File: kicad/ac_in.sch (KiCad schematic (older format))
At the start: 32 parts, among them J701 tblock, U702 R-783.3-1.0, U704 R-78E5.0-1.0, U705 AP2114H-1.2TRG1, U706 AP2114H-1.2TRG1

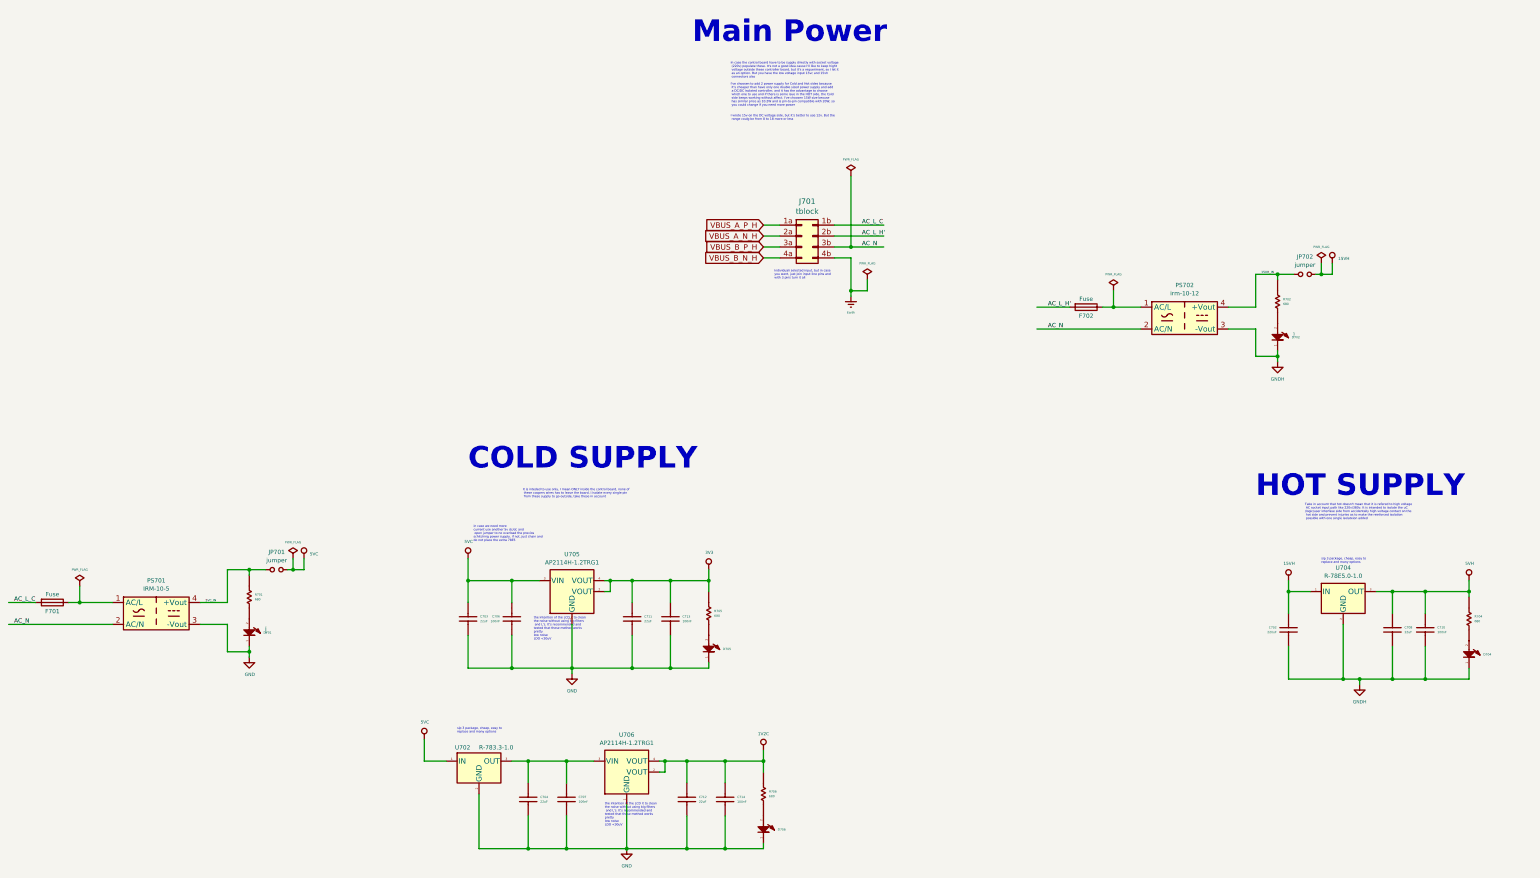
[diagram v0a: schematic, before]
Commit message: beginine routing... far far away
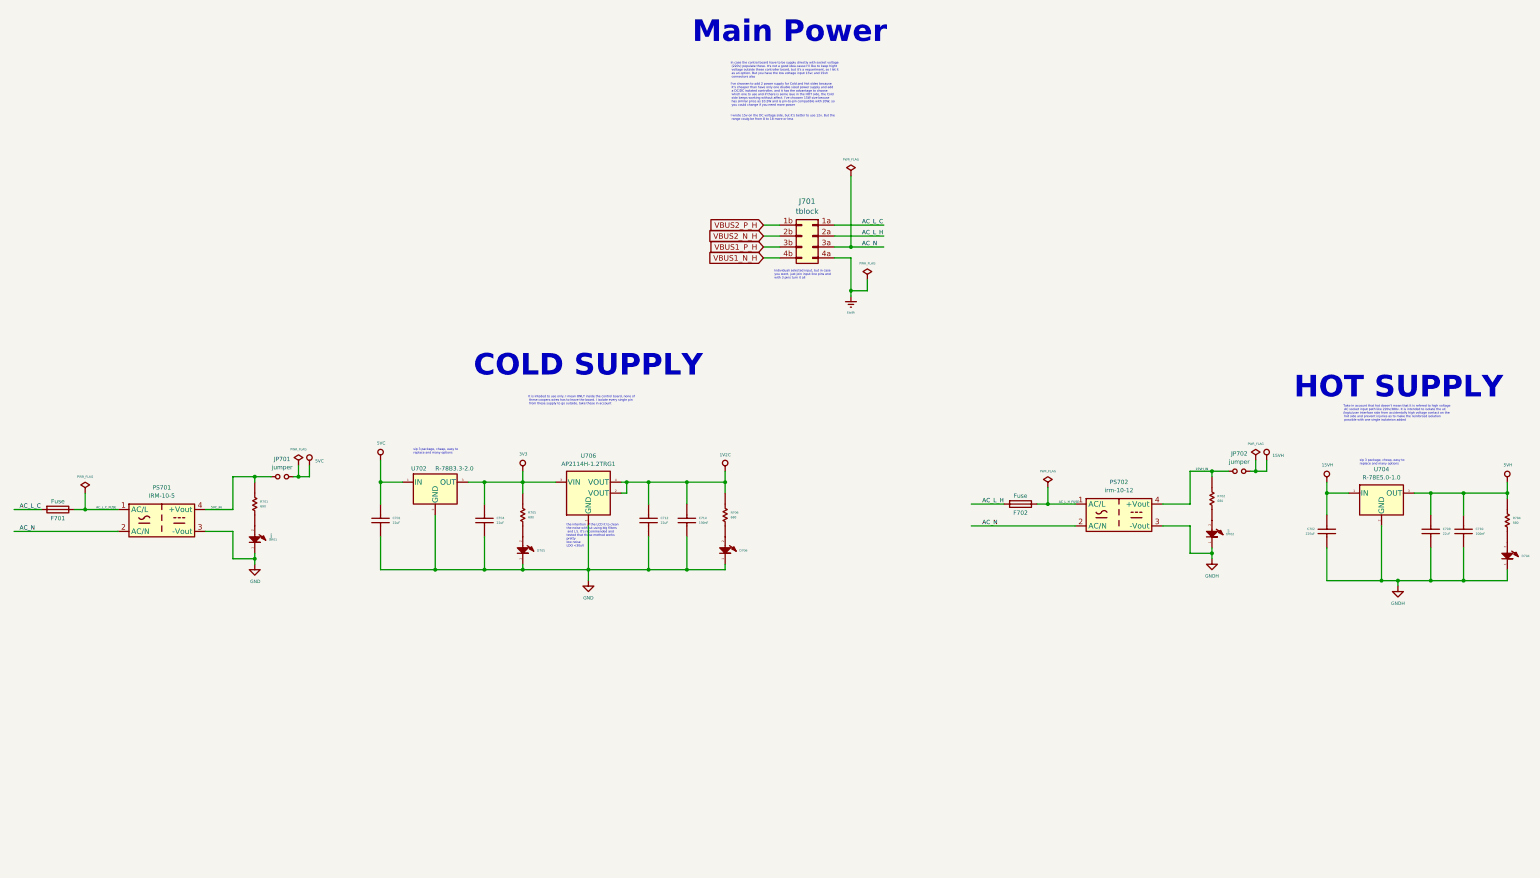
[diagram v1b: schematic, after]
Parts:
- removed C703, C711: 22uF, servo:C_0603_1608Metric, symbol servo:Capacitor
- removed C706, C707, C713: 100nF, servo:C_0603_1608Metric, symbol servo:Capacitor
- removed U705: AP2114H-1.2TRG1, Package_TO_SOT_SMD:SOT-223, symbol servo:AP2114
- added C701: 22uF, servo:C_0603_1608Metric, symbol servo:Capacitor
- U702: value R-783.3-1.0 -> R-78B3.3-2.0
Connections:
- net labels added: AC_L_C_FUSE, AC_L_H, AC_L_H_FUSE, VBUS1_N_H, VBUS1_P_H, VBUS2_N_H, VBUS2_P_H
- net labels removed: AC_L_H', VBUS_A_N_H, VBUS_A_P_H, VBUS_B_N_H, VBUS_B_P_H
- wire segments 130 -> 108
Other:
- note removed: "in case we need more \ncurrent use another 5v dc/dc and\n open jumper to no overload the previos \nschitching power supply. if not, just chain and \ndo not place the extra 78E5"
- moved on the sheet: C702, C704, C708, C710, C712, C714, D701, D702, D704, D705, D706, F701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

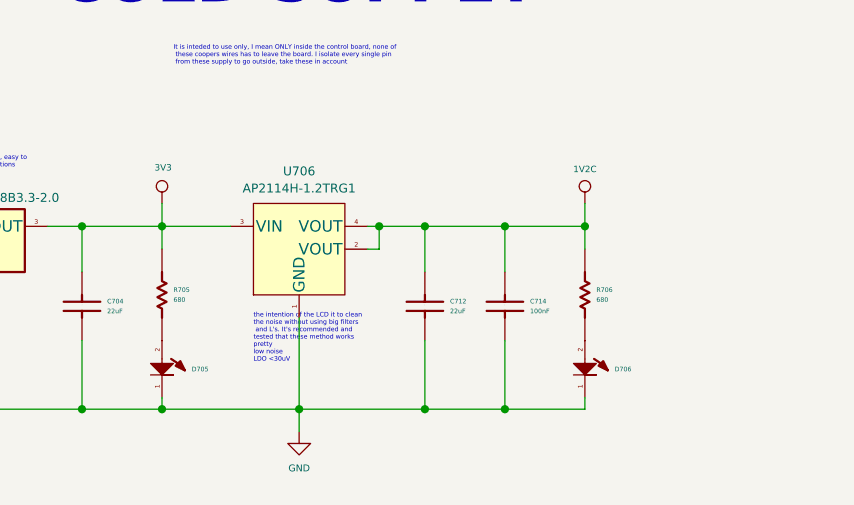
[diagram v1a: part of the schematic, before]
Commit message: touting....
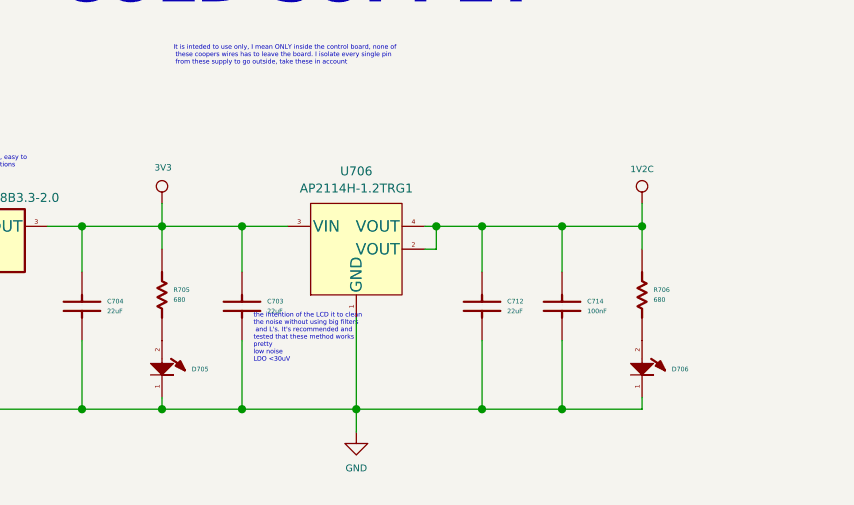
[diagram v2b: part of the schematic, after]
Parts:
- added C703: 22uF, servo:C_0603_1608Metric, symbol servo:Capacitor
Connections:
- wire segments 108 -> 112
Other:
- moved on the sheet: C712, C714, D706, R706, U706
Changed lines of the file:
@@
 L servo:1V2C #PWR0719
 U 1 1 5DDC3F59
-P 7850 5550
-F 0 "#PWR0719" H 7850 5350 20  0001 C CNN
-F 1 "1V2C" H 7850 5700 28  0000 C CNN
-F 2 "" H 7850 5550 50  0001 C CNN
-F 3 "" H 7850 5550 50  0001 C CNN
-	1    7850 5550
+P 8100 5550
+F 0 "#PWR0719" H 8100 5350 20  0001 C CNN
+F 1 "1V2C" H 8100 5700 28  0000 C CNN
+F 2 "" H 8100 5550 50  0001 C CNN
+F 3 "" H 8100 5550 50  0001 C CNN
+	1    8100 5550
 	1    0    0    -1
 $EndComp
@@
 	5200 5950 5200 6450
 Wire Wire Line
-	7850 5650 7850 5550
-Wire Wire Line
-	7850 5650 7850 5750
-Connection ~ 7850 5650
+	8100 5650 8100 5550
+Wire Wire Line
+	8100 5650 8100 5750
+Connection ~ 8100 5650
 $Comp
 L servo:Resistor R?
 U 1 1 5E18DDBA
-P 7850 5950
+P 8100 5950
 AR Path="/5EAA846A/5E18DDBA" Ref="R?"  Part="1"
 AR Path="/5DD76B18/5E18DDBA" Ref="R706"  Part="1"
-F 0 "R706" V 7828 6000 20  0000 L CNN
-F 1 "680" V 7871 6000 20  0000 L CNN
-F 2 "Resistor_SMD:R_0603_1608Metric" H 7350 5850 60  0001 C CNN
-F 3 "" H 7450 5950 60  0001 C CNN
-F 4 "680" V -4550 6350 60  0001 C CNN "ValueDisplayed"
-	1    7850 5950
+F 0 "R706" V 8078 6000 20  0000 L CNN
+F 1 "680" V 8121 6000 20  0000 L CNN
+F 2 "Resistor_SMD:R_0603_1608Metric" H 7600 5850 60  0001 C CNN
+F 3 "" H 7700 5950 60  0001 C CNN
+F 4 "680" V -4300 6350 60  0001 C CNN "ValueDisplayed"
+	1    8100 5950
 	0    1    1    0
 $EndComp
@@
 L servo:LED_A2_K1 D?
 U 1 1 5E18DDBB
-P 7850 6250
+P 8100 6250
 AR Path="/5EAA846A/5E18DDBB" Ref="D?"  Part="1"
 AR Path="/5DD76B18/5E18DDBB" Ref="D706"  Part="1"
-F 0 "D706" V 7875 6380 20  0000 L CNN
-F 1 "blue" H 7850 6400 16  0001 C CNN
-F 2 "servo:LED_0603_1608Metric" H 7650 6050 60  0001 C CNN
-F 3 "" H 7650 6050 60  0000 C CNN
-F 4 "red" V -4550 6150 60  0001 C CNN "VALUE"
-	1    7850 6250
-	0    1    1    0
-$EndComp
-Wire Wire Line
-	7850 6400 7850 6450
+F 0 "D706" V 8125 6380 20  0000 L CNN
+F 1 "blue" H 8100 6400 16  0001 C CNN
+F 2 "servo:LED_0603_1608Metric" H 7900 6050 60  0001 C CNN
+F 3 "" H 7900 6050 60  0000 C CNN
+F 4 "red" V -4300 6150 60  0001 C CNN "VALUE"
+	1    8100 6250
+	0    1    1    0
+$EndComp
+Wire Wire Line
+	8100 6400 8100 6450
 $Comp
 L servo:GND #PWR?
 U 1 1 5E286204
-P 6600 6550
+P 6850 6550
 AR Path="/5DCD812E/5E286204" Ref="#PWR?"  Part="1"
 AR Path="/5EAA846A/5E286204" Ref="#PWR?"  Part="1"
 AR Path="/5DD76B18/5E286204" Ref="#PWR0715"  Part="1"
-F 0 "#PWR0715" H 6605 6401 20  0001 C CNN
-F 1 "GND" H 6600 6392 30  0000 C CNN
-F 2 "" H 6600 6550 70  0000 C CNN
-F 3 "" H 6600 6550 70  0000 C CNN
-	1    6600 6550
+F 0 "#PWR0715" H 6855 6401 20  0001 C CNN
+F 1 "GND" H 6850 6392 30  0000 C CNN
+F 2 "" H 6850 6550 70  0000 C CNN
+F 3 "" H 6850 6550 70  0000 C CNN
+	1    6850 6550
 	1    0    0    -1
 $EndComp
@@
 L servo:Capacitor C?
 U 1 1 5E28620B
-P 7150 5950
+P 7400 5950
 AR Path="/5EAA846A/5E28620B" Ref="C?"  Part="1"
 AR Path="/5DD76B18/5E28620B" Ref="C712"  Part="1"
-F 0 "C712" V 7178 6060 20  0000 L CNN
-F 1 "22uF" V 7221 6060 20  0000 L CNN
-F 2 "servo:C_0603_1608Metric" H 7150 5850 60  0001 C CNN
-F 3 "" H 7150 5950 60  0000 C CNN
-F 4 "22uF" V -5850 6350 60  0001 C CNN "ValueDisplayed"
-	1    7150 5950
+F 0 "C712" V 7428 6060 20  0000 L CNN
+F 1 "22uF" V 7471 6060 20  0000 L CNN
+F 2 "servo:C_0603_1608Metric" H 7400 5850 60  0001 C CNN
+F 3 "" H 7400 5950 60  0000 C CNN
+F 4 "22uF" V -5600 6350 60  0001 C CNN "ValueDisplayed"
+	1    7400 5950
 	0    1    1    0
 $EndComp
@@
 L servo:Capacitor C?
 U 1 1 5E286219
-P 7500 5950
+P 7750 5950
 AR Path="/5EAA846A/5E286219" Ref="C?"  Part="1"
 AR Path="/5DD76B18/5E286219" Ref="C714"  Part="1"
-F 0 "C714" V 7528 6060 20  0000 L CNN
-F 1 "100nF" V 7571 6060 20  0000 L CNN
-F 2 "servo:C_0603_1608Metric" H 7500 5850 60  0001 C CNN
-F 3 "" H 7500 5950 60  0000 C CNN
-F 4 "22uF" V -5500 6350 60  0001 C CNN "ValueDisplayed"
-	1    7500 5950
+F 0 "C714" V 7778 6060 20  0000 L CNN
+F 1 "100nF" V 7821 6060 20  0000 L CNN
+F 2 "servo:C_0603_1608Metric" H 7750 5850 60  0001 C CNN
+F 3 "" H 7750 5950 60  0000 C CNN
+F 4 "22uF" V -5250 6350 60  0001 C CNN "ValueDisplayed"
+	1    7750 5950
 	0    1    1    0
 $EndComp
@@
 HOT SUPPLY
 Wire Wire Line
-	6900 5650 6950 5650
-Wire Wire Line
-	6900 5750 6950 5750
-Wire Wire Line
-	6950 5750 6950 5650
-Connection ~ 6950 5650
-Wire Wire Line
-	6600 6050 6600 6450
-Connection ~ 6600 6450
+	7150 5650 7200 5650
+Wire Wire Line
+	7150 5750 7200 5750
+Wire Wire Line
+	7200 5750 7200 5650
+Connection ~ 7200 5650
+Wire Wire Line
+	6850 6050 6850 6450
+Connection ~ 6850 6450
 Connection ~ 15000 5750
 Wire Wire Line
@@
 	5500 5650 5650 5650
 Wire Wire Line
-	6950 5650 7150 5650
+	7200 5650 7400 5650
 Wire Wire Line
 	5650 5850 5650 5650
@@
 L servo:AP2114 U706
 U 1 1 5E28622B
-P 6600 5750
-F 0 "U706" H 6600 6091 39  0000 C CNN
-F 1 "AP2114H-1.2TRG1" H 6600 6016 39  0000 C CNN
-F 2 "Package_TO_SOT_SMD:SOT-223" H 6700 6375 50  0001 C CNN
-F 3 "../doc/datasheets/AP2114.pdf" H 6650 6150 50  0001 C CNN
-	1    6600 5750
-	1    0    0    -1
-$EndComp
-Wire Wire Line
-	7150 6150 7150 6450
-Wire Wire Line
-	6600 6450 7150 6450
-Connection ~ 7150 6450
-Wire Wire Line
-	7150 6450 7500 6450
-Wire Wire Line
-	7500 6150 7500 6450
-Connection ~ 7500 6450
-Wire Wire Line
-	7500 6450 7850 6450
-Wire Wire Line
-	7150 5850 7150 5650
-Connection ~ 7150 5650
-Wire Wire Line
-	7500 5850 7500 5650
-Wire Wire Line
-	7150 5650 7500 5650
-Connection ~ 7500 5650
-Wire Wire Line
-	7500 5650 7850 5650
+P 6850 5750
+F 0 "U706" H 6850 6091 39  0000 C CNN
+F 1 "AP2114H-1.2TRG1" H 6850 6016 39  0000 C CNN
+F 2 "Package_TO_SOT_SMD:SOT-223" H 6950 6375 50  0001 C CNN
+F 3 "../doc/datasheets/AP2114.pdf" H 6900 6150 50  0001 C CNN
+	1    6850 5750
+	1    0    0    -1
+$EndComp
+Wire Wire Line
+	7400 6150 7400 6450
+Wire Wire Line
+	6850 6450 7400 6450
+Connection ~ 7400 6450
+Wire Wire Line
+	7400 6450 7750 6450
+Wire Wire Line
+	7750 6150 7750 6450
+Connection ~ 7750 6450
+Wire Wire Line
+	7750 6450 8100 6450
+Wire Wire Line
+	7400 5850 7400 5650
+Connection ~ 7400 5650
+Wire Wire Line
+	7750 5850 7750 5650
+Wire Wire Line
+	7400 5650 7750 5650
+Connection ~ 7750 5650
+Wire Wire Line
+	7750 5650 8100 5650
 Text Notes 6400 6250 0    20   ~ 0
 the intention of the LCD it to clean \nthe noise without using big filters\n and L's. It's recommended and \ntested that these method works \npretty\nlow noise \nLDO <30uV
@@
 Connection ~ 5650 6450
 Wire Wire Line
-	6000 5650 6300 5650
-Wire Wire Line
-	6600 6450 6000 6450
+	6000 5650 6350 5650
+Wire Wire Line
+	6850 6450 6350 6450
 Connection ~ 6000 6450
 Wire Wire Line
-	6600 6550 6600 6450
+	6850 6550 6850 6450
 Connection ~ 5200 6450
 Text Label 10900 5850 0    20   ~ 0
@@
 Wire Wire Line
 	8200 3400 8350 3400
+$Comp
+L servo:Capacitor C?
+U 1 1 5E2B77D4
+P 6350 5950
+AR Path="/5EAA846A/5E2B77D4" Ref="C?"  Part="1"
+AR Path="/5DD76B18/5E2B77D4" Ref="C703"  Part="1"
+F 0 "C703" V 6378 6060 20  0000 L CNN
+F 1 "22uF" V 6421 6060 20  0000 L CNN
+F 2 "servo:C_0603_1608Metric" H 6350 5850 60  0001 C CNN
+F 3 "" H 6350 5950 60  0000 C CNN
+F 4 "22uF" V -6650 6350 60  0001 C CNN "ValueDisplayed"
+	1    6350 5950
+	0    1    1    0
+$EndComp
+Wire Wire Line
+	6350 5850 6350 5650
+Connection ~ 6350 5650
+Wire Wire Line
+	6350 5650 6550 5650
+Wire Wire Line
+	6350 6150 6350 6450
+Connection ~ 6350 6450
+Wire Wire Line
+	6350 6450 6000 6450
 $EndSCHEMATC
